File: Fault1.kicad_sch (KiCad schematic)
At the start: 15 parts

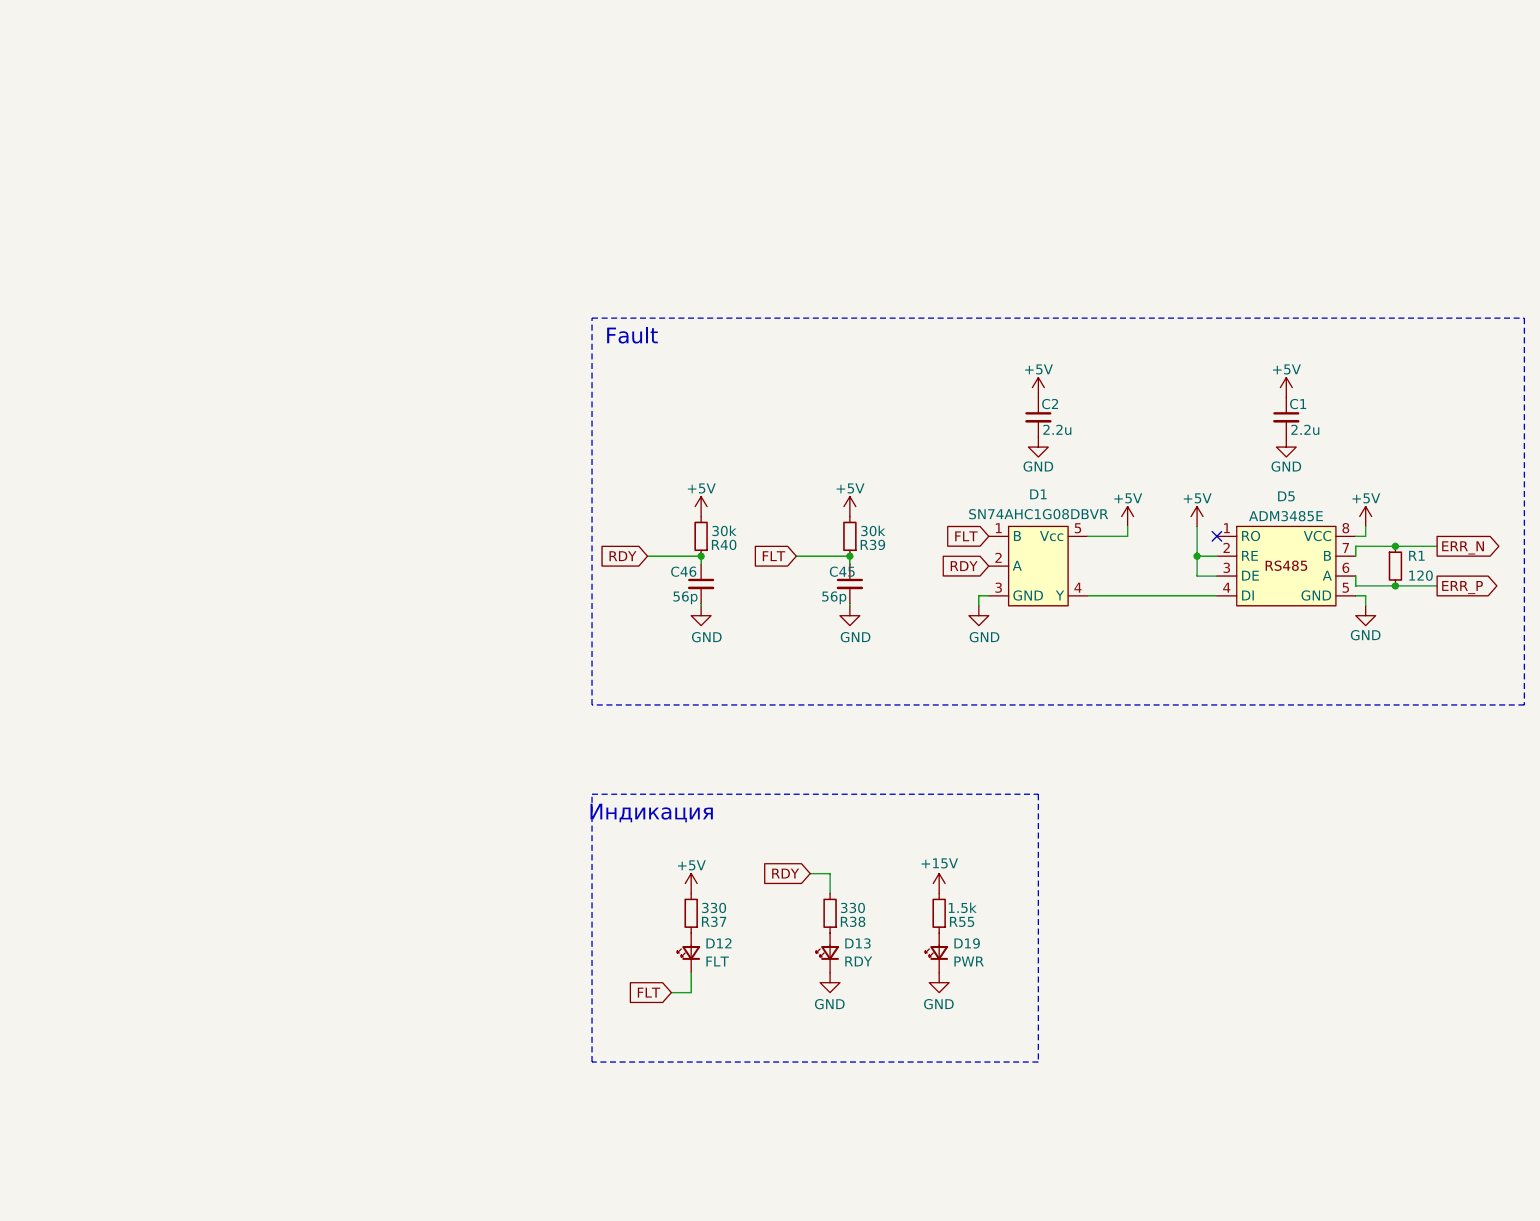
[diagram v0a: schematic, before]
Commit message: Развел вторую стойку
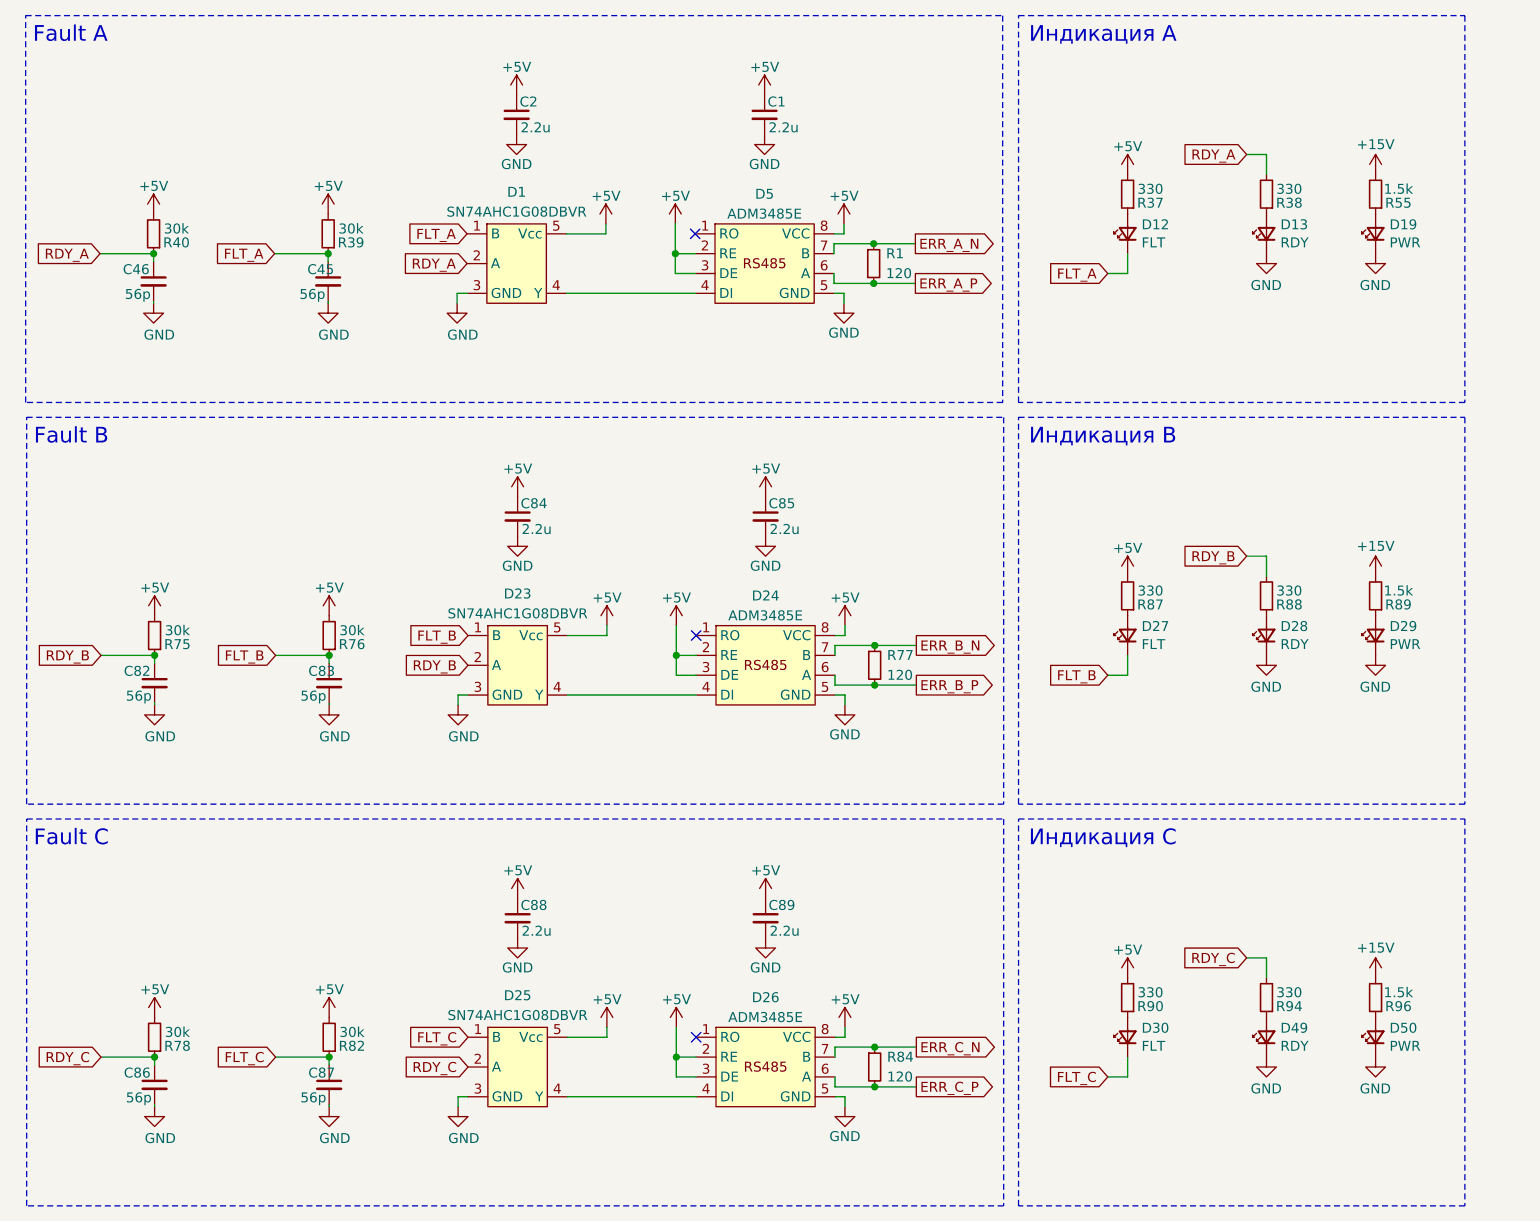
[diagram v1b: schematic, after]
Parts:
- added C82, C83, C86, C87: 56p, Capacitor_SMD:C_0805_2012Metric_Pad1.18x1.45mm_HandSolder, symbol Device:C_Small
- added C84, C85, C88, C89: 2.2u, Capacitor_SMD:C_0805_2012Metric_Pad1.18x1.45mm_HandSolder, symbol Device:C_Small
- added D23, D25: SN74AHC1G08DBVR, Package_TO_SOT_SMD:SOT-23-5_HandSoldering, symbol Logic_My:MC74VHC1GT08DTT1G
- added D24, D26: ADM3485E, Package_SO:SOIC-8_3.9x4.9mm_P1.27mm, symbol Interface_My:ADM3485E_1
- added D27, D30: FLT, LED_SMD:LED_0805_2012Metric_Pad1.15x1.40mm_HandSolder, symbol Device:LED_Small
- added D28, D49: RDY, LED_SMD:LED_0805_2012Metric_Pad1.15x1.40mm_HandSolder, symbol Device:LED_Small
- added D29, D50: PWR, LED_SMD:LED_0805_2012Metric_Pad1.15x1.40mm_HandSolder, symbol Device:LED_Small
- added R75, R76, R78, R82: 30k, Resistor_SMD:R_0805_2012Metric_Pad1.20x1.40mm_HandSolder, symbol Device:R_Small
- added R77, R84: 120, Resistor_SMD:R_0805_2012Metric_Pad1.20x1.40mm_HandSolder, symbol Device:R_Small
- added R87, R88, R90, R94: 330, Resistor_SMD:R_0805_2012Metric_Pad1.20x1.40mm_HandSolder, symbol Device:R_Small
- added R89, R96: 1.5k, Resistor_SMD:R_0805_2012Metric_Pad1.20x1.40mm_HandSolder, symbol Device:R_Small
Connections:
- net +15V: now also R89.2, R96.2
- net +5V: now also C84.1, C85.1, C88.1, C89.1, D23.5 (Vcc), D24.2 (RE), D24.3 (DE), D24.8 (VCC), D25.5 (Vcc), D26.2 (RE), D26.3 (DE), D26.8 (VCC), R75.2, R76.2, R78.2, R82.2, R87.2, R90.2
- net GND: now also C82.2, C83.2, C84.2, C85.2, C86.2, C87.2, C88.2, C89.2, D23.3 (GND), D24.5 (GND), D25.3 (GND), D26.5 (GND), D28.1 (K), D29.1 (K), D49.1 (K), D50.1 (K)
- net ERR_N renamed ERR_A_N
- net ERR_P renamed ERR_A_P
- net FLT renamed FLT_A
- net RDY renamed RDY_A
- new net: D30.2 (A), R90.1
- new net: D49.2 (A), R94.1
- new net: D25.4 (Y), D26.4 (DI)
- new net: D50.2 (A), R96.1
- new net: D29.2 (A), R89.1
- new net: D28.2 (A), R88.1
- new net: D27.2 (A), R87.1
- new net: D23.4 (Y), D24.4 (DI)
- new net ERR_B_N: D24.7 (B), R77.1
- new net ERR_B_P: D24.6 (A), R77.2
- new net ERR_C_N: D26.7 (B), R84.1
- new net ERR_C_P: D26.6 (A), R84.2
- new net FLT_B: C83.1, D23.1 (B), D27.1 (K), R76.1
- new net FLT_C: C87.1, D25.1 (B), D30.1 (K), R82.1
- new net RDY_B: C82.1, D23.2 (A), R75.1, R88.2
- new net RDY_C: C86.1, D25.2 (A), R78.1, R94.2
- no-connect marks 1 -> 3
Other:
- note added: "Fault A"
- note added: "Fault B"
- note added: "Fault C"
- note added: "Индикация A"
- note added: "Индикация B"
- note added: "Индикация C"
- note removed: "Fault"
- note removed: "Индикация"
- moved on the sheet: C1, C2, C45, C46, D1, D12, D13, D19, D5, R1, R37, R38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
